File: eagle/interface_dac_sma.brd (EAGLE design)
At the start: 109.5 x 126 mm, 27 parts, among them IC1 ISO1540, X1 BU-SMA-V

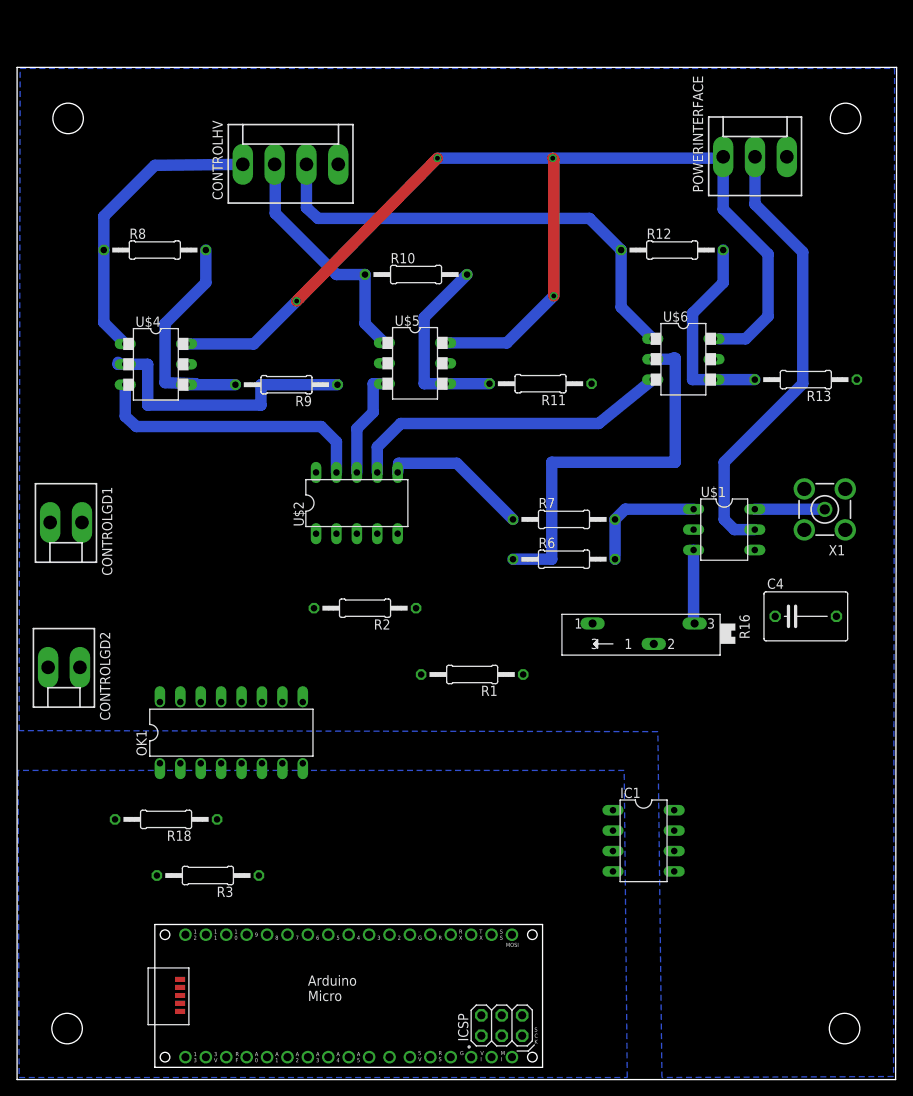
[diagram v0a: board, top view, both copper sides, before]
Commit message: board tweak
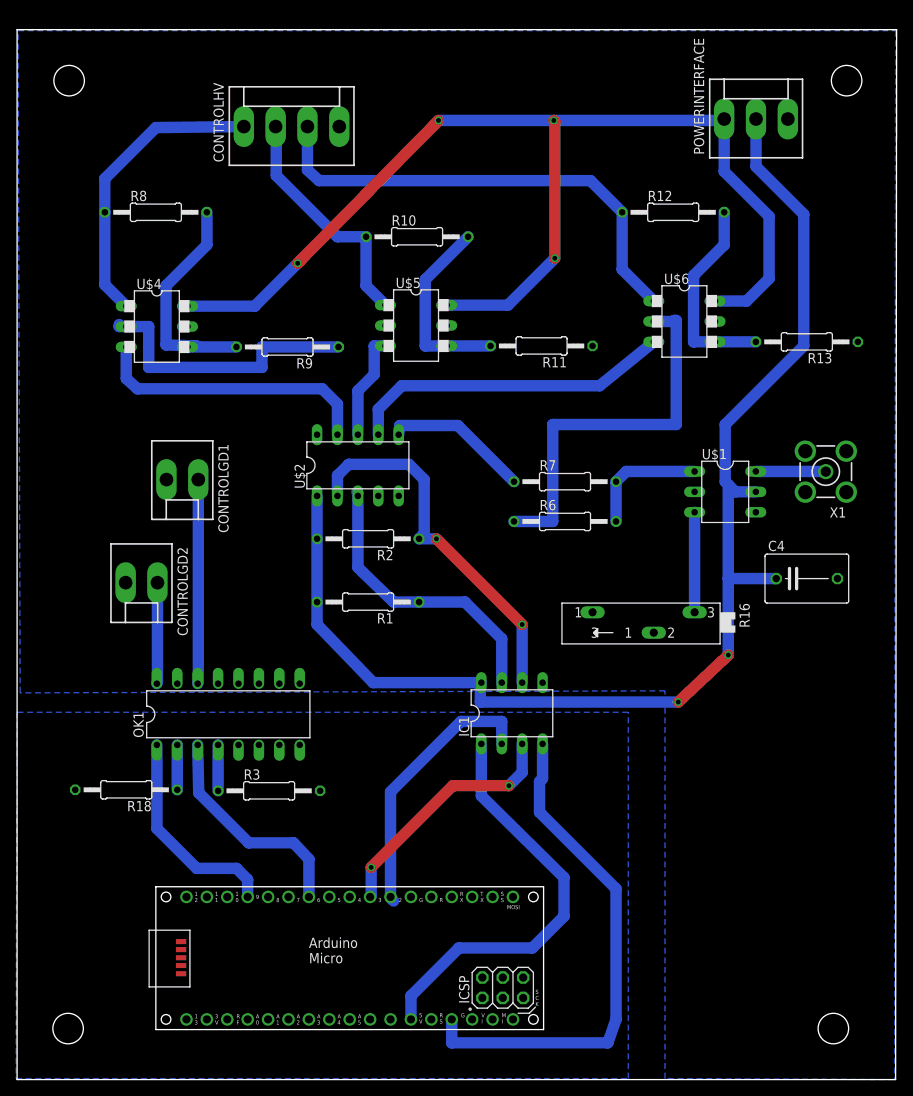
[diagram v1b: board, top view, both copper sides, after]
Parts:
- moved IC1 22.8 mm to (61.6, 45.6), turned to 0 degrees
- moved R1 15.8 mm to (43.7, 59.4)
- moved CONTROLGD1 15.4 mm to (20.6, 74.7)
- moved CONTROLGD2 14.3 mm to (15.5, 61.8)
- moved R3 13.0 mm to (31.4, 35.9), turned to 0 degrees
- moved R2 8.64 mm to (43.7, 67.3)
- moved R18 6.17 mm to (13.6, 36.1)
- moved R9 4.70 mm to (33.7, 91.2)
- moved PCB1 4.70 mm to (17.3, 6.22)
- moved C4 4.70 mm to (98.3, 62.4)
- moved CONTROLHV 4.70 mm to (34.2, 118.6)
- moved POWERINTERFACE 4.70 mm to (92.0, 119.6)
- moved R10 4.70 mm to (49.8, 104.9)
- moved R11 4.70 mm to (65.3, 91.3)
- moved R12 4.70 mm to (81.7, 108.0)
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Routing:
- net VCC: track 56.0 -> 158.3 mm, vias 0 -> 2
- net AGND: track 0.00 -> 63.8 mm
- net A+5: track 0.00 -> 51.8 mm
- net SCL_OUT: track 0.00 -> 46.8 mm, vias 0 -> 2
- net SDA_OUT: track 0.00 -> 36.5 mm
- net SDA: track 0.00 -> 34.0 mm
- net SCL: track 0.00 -> 31.0 mm, vias 0 -> 2
- net PWM6: track 0.00 -> 27.8 mm
- net PWM9: track 0.00 -> 26.5 mm
- net ENSW1: track 0.00 -> 25.4 mm
- net ENSW2: track 0.00 -> 12.6 mm
- net N$10: track 0.00 -> 5.71 mm
- net N$7: track 0.00 -> 5.59 mm
- net N$12: track 9.20 -> 12.4 mm
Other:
- board size 109.5 x 126 mm -> 109.5 x 130.7 mm
